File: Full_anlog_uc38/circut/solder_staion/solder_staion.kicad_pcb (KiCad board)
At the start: 2 copper layers, 23.6 x 25.9 mm, 24 parts, among them J1 Screw_Terminal_01x02, J3 Conn_01x01_Pin, J4 Conn_01x01_Pin, J5 Conn_01x01_Pin, J6 Conn_01x01_Pin, Q2 Si4162DY, U1 UC3842_SOIC8

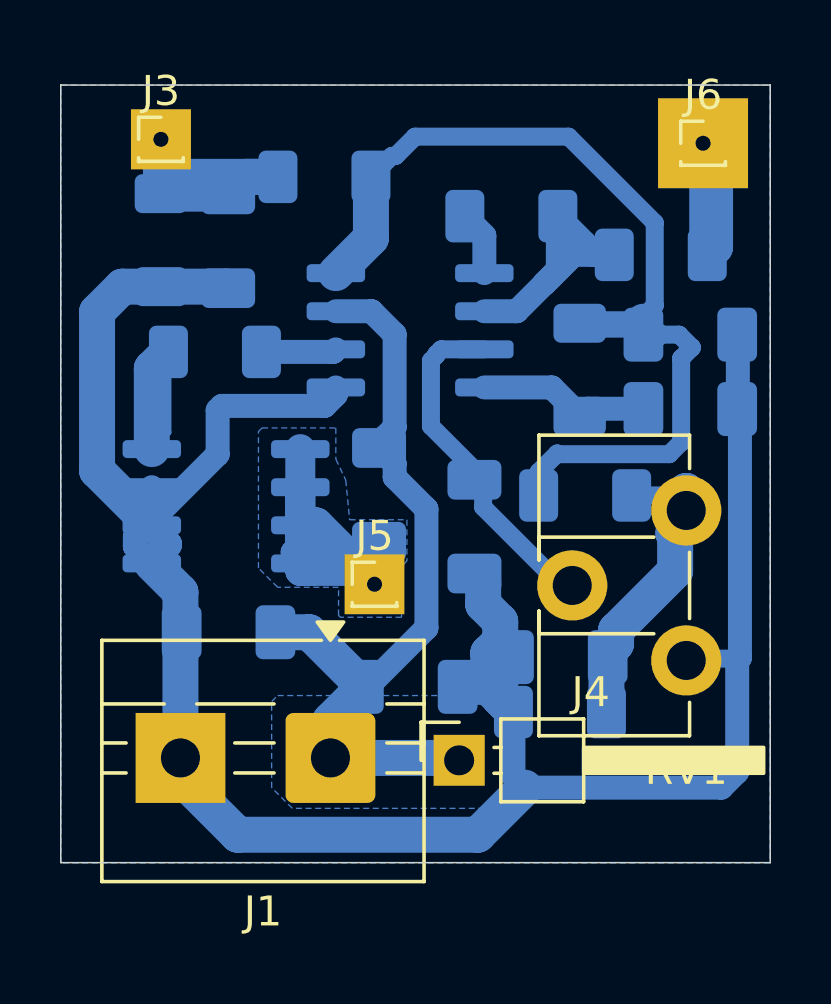
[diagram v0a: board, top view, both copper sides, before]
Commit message: k
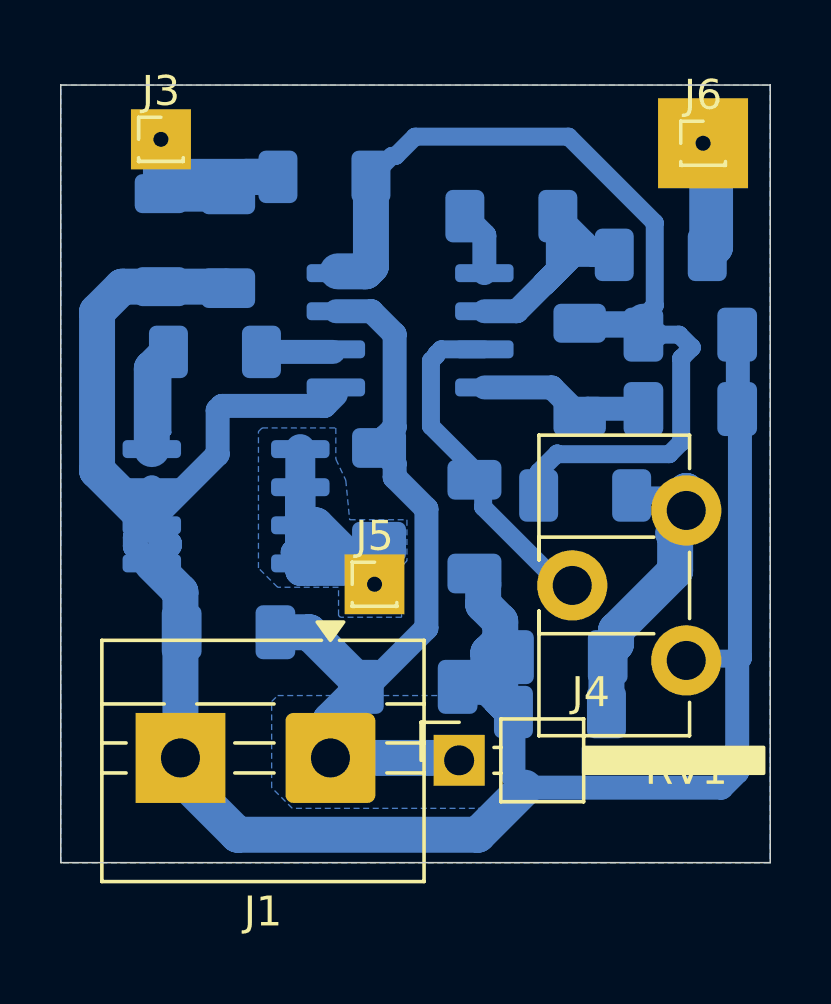
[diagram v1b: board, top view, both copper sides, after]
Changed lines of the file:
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@@
-	)
-	(segment
-		(start 215.845 96.905)
-		(end 216.22 96.53)
-		(width 0.8)
-		(layer "B.Cu")
-		(net 2)
 	)
 	(segment
@@
 	)
 	(segment
-		(start 212.28 98.52)
-		(end 212.28 97.05)
-		(width 0.8)
-		(layer "B.Cu")
-		(net 2)
-	)
-	(segment
 		(start 210.085 100.885)
 		(end 208.26 99.06)
@@
 	)
 	(segment
+		(start 209.52 101.59)
+		(end 210.085 102.155)
+		(width 0.8)
+		(layer "B.Cu")
+		(net 2)
+	)
+	(segment
 		(start 221.13 102.7825)
 		(end 220.84 102.4925)
@@
 	)
 	(segment
-		(start 212.28 97.05)
-		(end 212.425 96.905)
-		(width 0.8)
-		(layer "B.Cu")
-		(net 2)
-	)
-	(segment
 		(start 220.95 111.2)
 		(end 222.52 109.63)
@@
 	)
 	(segment
-		(start 214.52 97.15)
-		(end 215.6 97.15)
+		(start 215.6 97.15)
+		(end 214.52 97.15)
 		(width 0.2)
 		(layer "B.Cu")
@@
 	)
 	(segment
-		(start 209.52 101.28)
-		(end 212.28 98.52)
+		(start 212.28 98.52)
+		(end 209.52 101.28)
 		(width 0.8)
 		(layer "B.Cu")
@@
 	)
 	(segment
-		(start 215.6 97.15)
-		(end 216.22 96.53)
-		(width 0.2)
-		(layer "B.Cu")
-		(net 2)
-	)
-	(segment
 		(start 210.085 100.885)
 		(end 210.085 99.615)
@@
 	)
 	(segment
-		(start 212.425 96.905)
-		(end 215.845 96.905)
-		(width 0.8)
-		(layer "B.Cu")
-		(net 2)
-	)
-	(segment
-		(start 209.52 101.59)
-		(end 209.52 101.28)
+		(start 209.52 101.28)
+		(end 209.52 101.59)
 		(width 0.8)
 		(layer "B.Cu")
@@
 	)
 	(segment
+		(start 212.28 97.05)
+		(end 212.28 98.52)
+		(width 0.8)
+		(layer "B.Cu")
+		(net 2)
+	)
+	(segment
 		(start 221.7 104.09)
 		(end 221.13 103.52)
@@
 	)
 	(segment
-		(start 210.085 102.155)
-		(end 209.52 101.59)
-		(width 0.8)
-		(layer "B.Cu")
-		(net 2)
-	)
-	(segment
 		(start 211.04 103.11)
 		(end 210.085 102.155)
@@
 	)
 	(segment
+		(start 212.425 96.905)
+		(end 212.28 97.05)
+		(width 0.8)
+		(layer "B.Cu")
+		(net 2)
+	)
+	(segment
+		(start 216.22 96.53)
+		(end 215.6 97.15)
+		(width 0.2)
+		(layer "B.Cu")
+		(net 2)
+	)
+	(segment
 		(start 221.7 106.67)
 		(end 221.7 104.74)
@@
 	)
 	(segment
+		(start 215.845 96.905)
+		(end 212.425 96.905)
+		(width 0.8)
+		(layer "B.Cu")
+		(net 2)
+	)
+	(segment
 		(start 222.14 107.11)
 		(end 222.14 109.25)
@@
 	(segment
 		(start 216.22 96.53)
-		(end 216.22 96.29)
+		(end 215.845 96.905)
 		(width 0.8)
 		(layer "B.Cu")
@@
 	)
 	(segment
+		(start 217.21 92.42)
+		(end 216.28 92.42)
+		(width 1.2)
+		(layer "B.Cu")
+		(net 3)
+	)
+	(segment
 		(start 226.4725 94.53)
 		(end 226.4725 93.9375)
@@
 	)
 	(segment
-		(start 217.39 91.31)
-		(end 216.22 92.48)
-		(width 1.2)
-		(layer "B.Cu")
-		(net 3)
-	)
-	(segment
-		(start 217.39 89.27)
-		(end 217.39 91.31)
-		(width 1.2)
-		(layer "B.Cu")
-		(net 3)
-	)
-	(segment
 		(start 227.73 98.12)
 		(end 227.73 95.32)
@@
 		(end 226.85 90.8)
 		(width 0.6)
+		(layer "B.Cu")
+		(net 3)
+	)
+	(segment
+		(start 217.39 89.27)
+		(end 217.39 92.24)
+		(width 1.2)
+		(layer "B.Cu")
+		(net 3)
+	)
+	(segment
+		(start 217.39 92.24)
+		(end 217.21 92.42)
+		(width 1.2)
 		(layer "B.Cu")
 		(net 3)
@@
 		(layer "B.Cu")
 		(net 12)
-	)
-	(segment
-		(start 216.135 95.105)
-		(end 216.22 95.02)
-		(width 0.8)
-		(layer "B.Cu")
-		(net 12)
